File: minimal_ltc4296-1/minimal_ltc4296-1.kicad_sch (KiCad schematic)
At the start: 19 parts, among them Q1 100.0 V, U1 LTC4296AUK-1-PBF

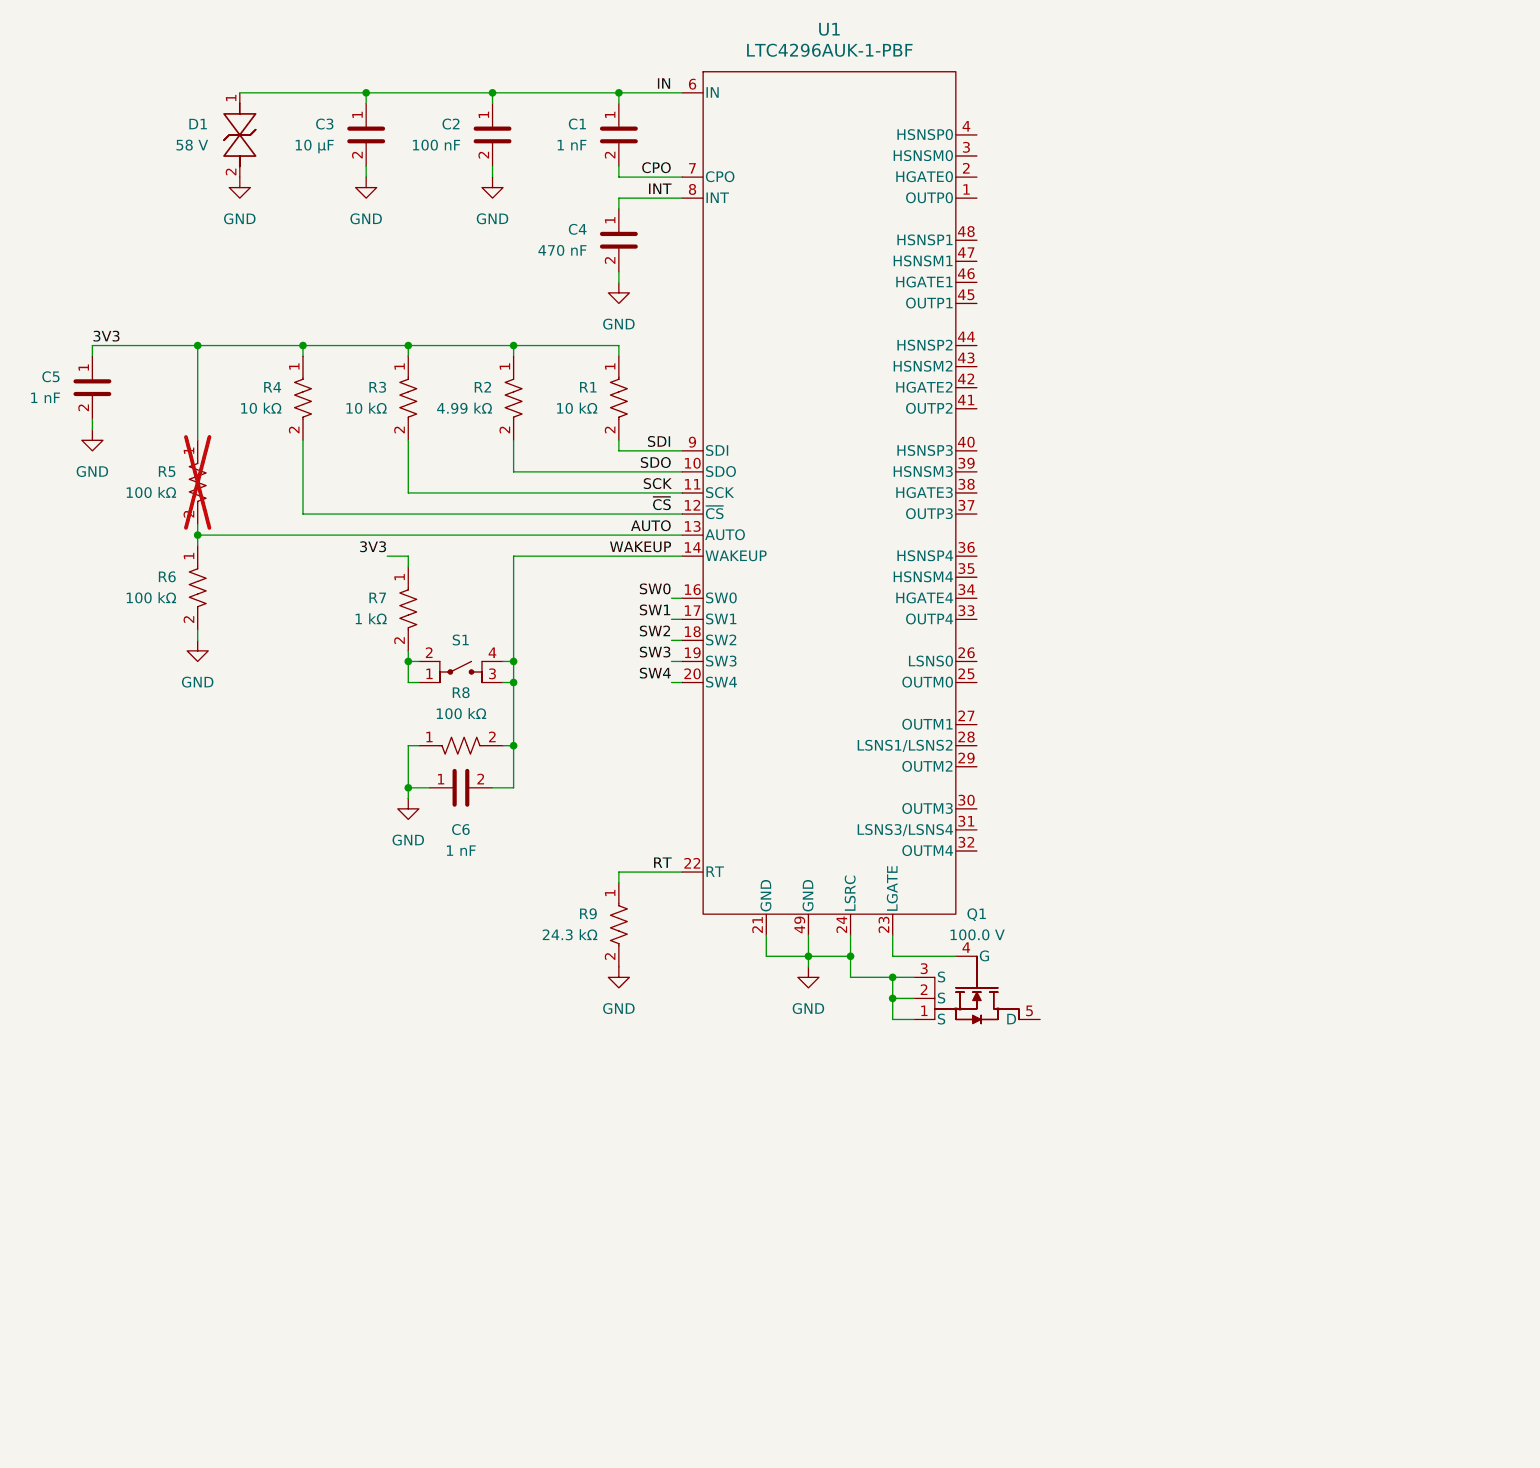
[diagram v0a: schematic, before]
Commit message: Update KiCAD schematic and PCB files
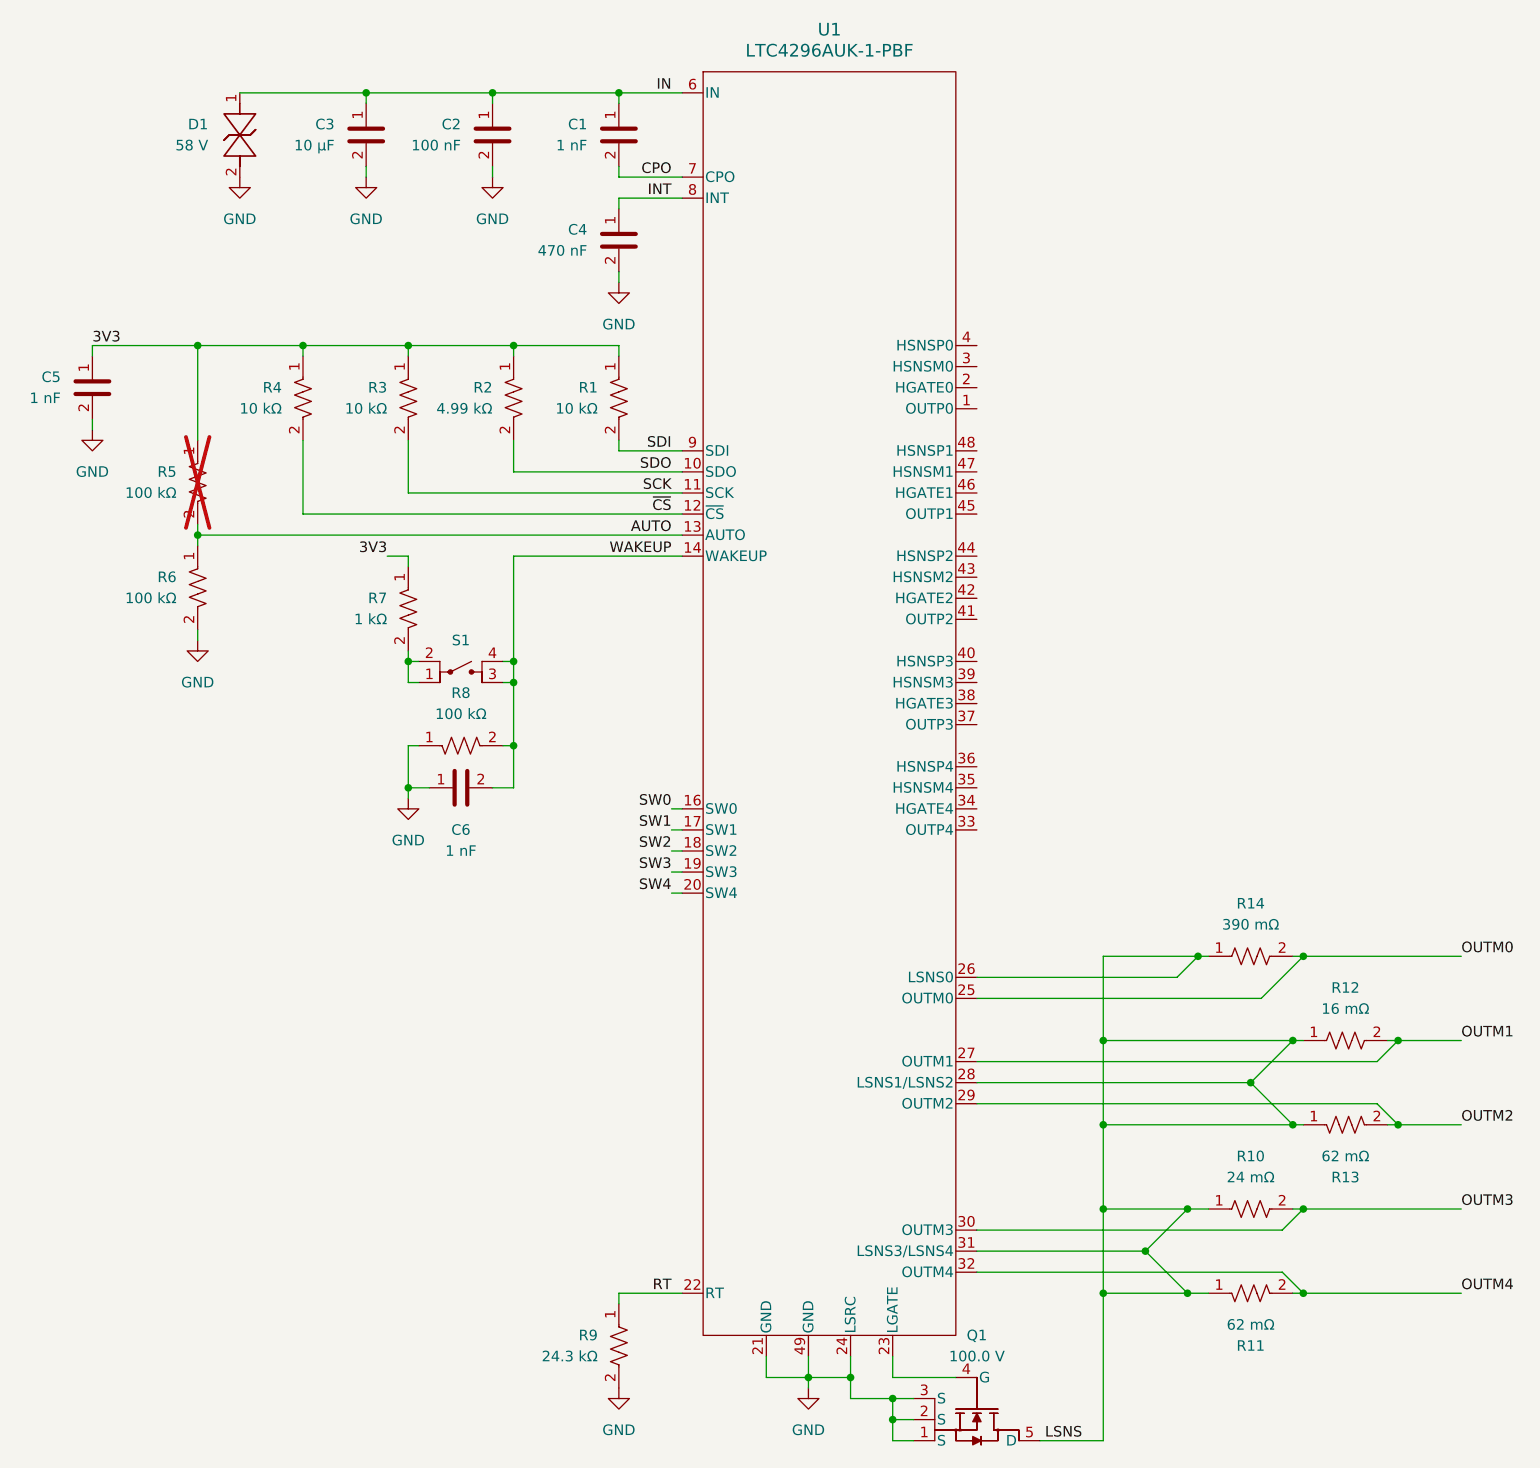
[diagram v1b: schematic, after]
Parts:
- added R10: 24 mΩ, resistor_footprints:R_0612_1632Metric, symbol RESISTORS_ERJ-B2CF_DATA_BASE:R_ERJ-B2CFR024V
- added R11, R13: 62 mΩ, resistor_footprints:R_0612_1632Metric, symbol RESISTORS_PRL1632-_DATA_BASE:R_PRL1632-R062-F-T1
- added R12: 16 mΩ, resistor_footprints:R_0612_1632Metric, symbol RESISTORS_PRL1632-_DATA_BASE:R_PRL1632-R016-F-T1
- added R14: 390 mΩ, resistor_footprints:R_0612_1632Metric, symbol RESISTORS_ERJ-B2BF_DATA_BASE:R_ERJ-B2BFR39V
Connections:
- net OUTM0: now reaches U1.25 (OUTM0)
- net OUTM0: now also R14.2
- net LSNS: now reaches U1.26 (LSNS0)
- net LSNS: now also Q1.5 (D), U1.28 (LSNS1/LSNS2), U1.31 (LSNS3/LSNS4), R10.1, R11.1, R12.1, R13.1, R14.1
- net OUTM1: now reaches U1.27 (OUTM1)
- net OUTM1: now also R12.2
- net OUTM2: now reaches U1.29 (OUTM2)
- net OUTM2: now also R13.2
- net OUTM3: now reaches U1.30 (OUTM3)
- net OUTM3: now also R10.2
- net OUTM4: now reaches U1.32 (OUTM4)
- net OUTM4: now also R11.2
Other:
- moved on the sheet: Q1, R9, U1
